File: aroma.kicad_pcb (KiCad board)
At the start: 4 copper layers, 96 x 44 mm, 108 parts, among them IC1 ESP32-WROOM-32E-N8R2, J1 USB4105-GF-A, J2 691137710003, J3 691137710002, J4 691137710002, J5 691137710002, J6 691137710002, J7 691137710002, J8 691137710002, J9 691137710002, Q1 SS8050, Q2 SS8050, SW1 1825910-6, SW2 1825910-6, SW3 JS5208, U1 FT231XS, U10 BSR802NL6327HTSA1, U11 BSR802NL6327HTSA1, U12 BSR802NL6327HTSA1, U2 ADP1613ARMZ-R7, U3 AMS1117-3.3, U4 74HC14, U6 BSR802NL6327HTSA1, U7 BSR802NL6327HTSA1, U8 BSR802NL6327HTSA1, U9 BSR802NL6327HTSA1

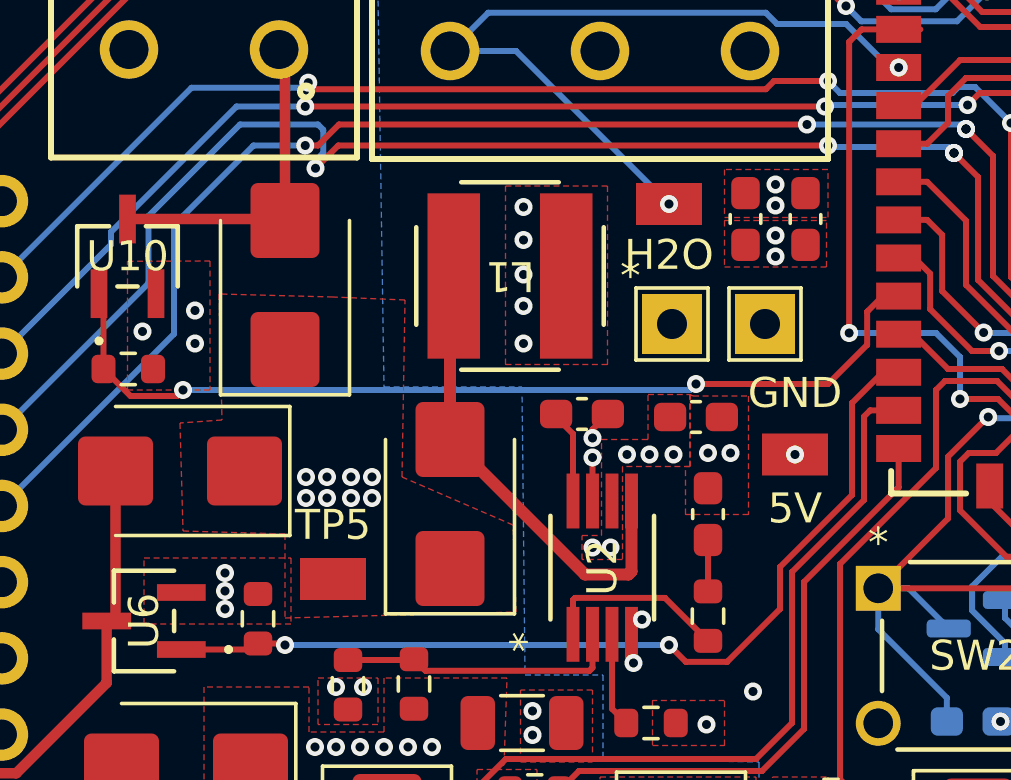
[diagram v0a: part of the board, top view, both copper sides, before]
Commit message: fix prelims
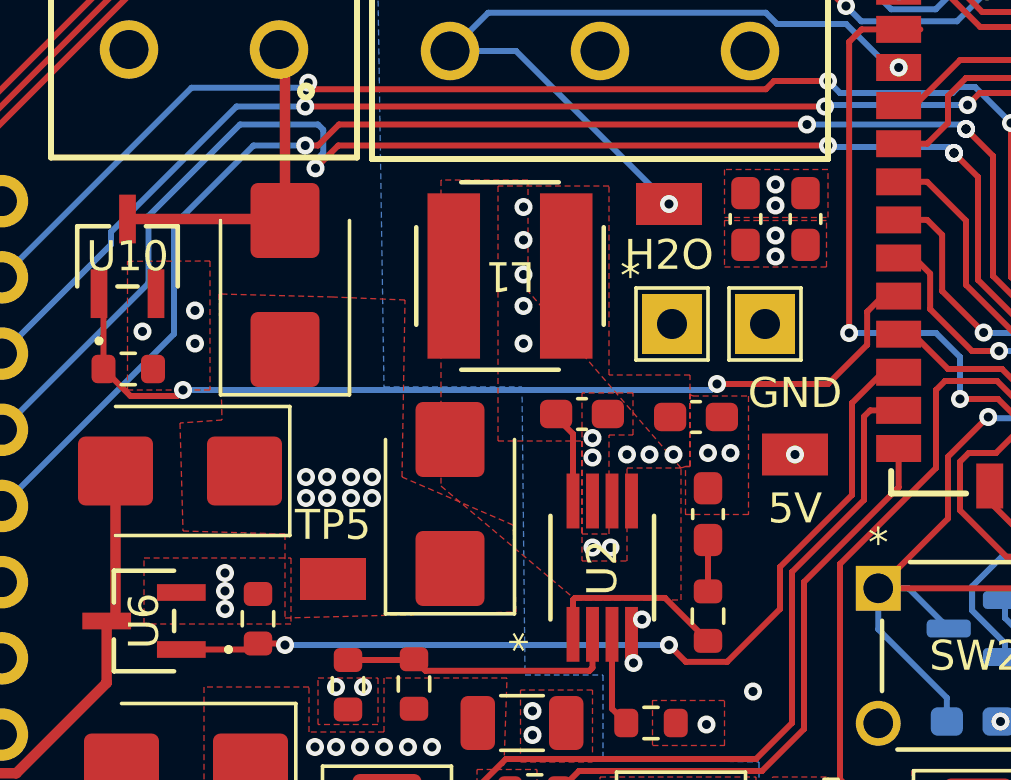
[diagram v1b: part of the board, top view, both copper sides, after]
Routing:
- net Net-(D4-A): track 15.8 -> 0.18 mm
- net GND: track 38.4 -> 35.9 mm
- added copper zone on F.Cu, net Net-(D4-A)
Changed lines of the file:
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@@
 	)
 	(segment
-		(start 138.65 96.45)
-		(end 138.65 97.899998)
-		(width 0.2)
-		(layer "F.Cu")
-		(net 1)
-	)
-	(segment
 		(start 126.250001 100.949999)
 		(end 126.4 100.8)
@@
 	)
 	(segment
-		(start 138.65 95.8)
-		(end 138.65 95.5125)
-		(width 0.2)
-		(layer "F.Cu")
-		(net 1)
-	)
-	(segment
 		(start 151.89 97.93)
 		(end 153.321299 99.361299)
@@
 	)
 	(segment
-		(start 138.65 95.5125)
-		(end 139.1625 95)
-		(width 0.2)
-		(layer "F.Cu")
-		(net 1)
-	)
-	(segment
 		(start 166.4875 100.860599)
 		(end 166.4875 102.6875)
@@
 	)
 	(segment
-		(start 133.9 95.85)
-		(end 133.9 90.525)
-		(width 0.4)
-		(layer "F.Cu")
-		(net 19)
-	)
-	(segment
-		(start 138.4 100.35)
-		(end 133.9 95.85)
-		(width 0.4)
-		(layer "F.Cu")
-		(net 19)
-	)
-	(segment
-		(start 139.949998 97.9)
-		(end 139.949998 100.250002)
-		(width 0.4)
-		(layer "F.Cu")
-		(net 19)
-	)
-	(segment
-		(start 139.85 100.35)
-		(end 138.4 100.35)
-		(width 0.4)
-		(layer "F.Cu")
-		(net 19)
-	)
-	(segment
 		(start 133.9 90.525)
 		(end 134.025 90.4)
@@
 	)
 	(segment
-		(start 139.949998 100.250002)
-		(end 139.85 100.35)
-		(width 0.4)
-		(layer "F.Cu")
-		(net 19)
-	)
-	(segment
 		(start 122.74 96.89)
 		(end 122.75 96.9)
@@
 	)
 	(segment
-		(start 142.1 94)
-		(end 146.5 94)
+		(start 125 94.2)
+		(end 124.8 94.4)
 		(width 0.2)
 		(layer "F.Cu")
@@
 	)
 	(segment
-		(start 125 94.2)
-		(end 124.8 94.4)
+		(start 147.805 92.695)
+		(end 147.805 91.59)
 		(width 0.2)
 		(layer "F.Cu")
@@
 	)
 	(segment
-		(start 147.805 91.59)
-		(end 148.325 91.07)
+		(start 142.8 94)
+		(end 146.5 94)
 		(width 0.2)
 		(layer "F.Cu")
@@
 	)
 	(segment
-		(start 124.8 94.4)
-		(end 123.25 94.4)
+		(start 147.805 91.59)
+		(end 148.325 91.07)
 		(width 0.2)
 		(layer "F.Cu")
@@
 	)
 	(segment
-		(start 148.325 91.07)
-		(end 148.855 91.07)
+		(start 124.8 94.4)
+		(end 123.25 94.4)
 		(width 0.2)
 		(layer "F.Cu")
@@
 	)
 	(segment
-		(start 122.35 91.1392)
-		(end 122.2 90.9892)
+		(start 146.5 94)
+		(end 147.805 92.695)
 		(width 0.2)
 		(layer "F.Cu")
@@
 	)
 	(segment
-		(start 147.805 92.695)
-		(end 147.805 91.59)
+		(start 122.35 91.1392)
+		(end 122.2 90.9892)
 		(width 0.2)
 		(layer "F.Cu")
@@
 	)
 	(segment
-		(start 146.5 94)
-		(end 147.805 92.695)
+		(start 148.325 91.07)
+		(end 148.855 91.07)
 		(width 0.2)
 		(layer "F.Cu")
@@
 	)
 	(via
-		(at 142.1 94)
+		(at 142.8 94)
 		(size 0.6)
 		(drill 0.3)
@@
 	)
 	(segment
-		(start 142.1 94)
-		(end 141.9 94.2)
+		(start 142.8 94)
+		(end 142.6 94.2)
 		(width 0.2)
 		(layer "B.Cu")
@@
 	)
 	(segment
-		(start 141.9 94.2)
+		(start 142.6 94.2)
 		(end 125 94.2)
 		(width 0.2)
@@
 	)
 	(zone
+		(net 1)
+		(net_name "GND")
+		(layer "F.Cu")
+		(hatch edge 0.5)
+		(priority 2)
+		(connect_pads yes
+			(clearance 0.25)
+		)
+		(min_thickness 0.25)
+		(filled_areas_thickness no)
+		(fill yes
+			(thermal_gap 0.5)
+			(thermal_bridge_width 0.5)
+		)
+		(polygon
+			(pts
+				(xy 140 94.3) (xy 138.3 94.3) (xy 138.3 99) (xy 139.2 99) (xy 139.2 95.7) (xy 140 95.7)
+			)
+		)
+	)
+	(zone
 		(net 6)
 		(net_name "+5V")
@@
 	)
 	(zone
-		(net 6)
-		(net_name "+5V")
-		(layer "F.Cu")
-		(hatch edge 0.5)
-		(priority 16)
-		(connect_pads yes
-			(clearance 0.25)
-		)
-		(min_thickness 0.2)
-		(filled_areas_thickness no)
-		(fill yes
-			(thermal_gap 0.5)
-			(thermal_bridge_width 0.5)
-		)
-		(polygon
-			(pts
-				(xy 135.75 87.4) (xy 139.15 87.4) (xy 139.15 93.35) (xy 135.75 93.35)
-			)
-		)
-	)
-	(zone
 		(net 1)
 		(net_name "GND")
@@
 	)
 	(zone
+		(net 19)
+		(net_name "Net-(D4-A)")
+		(layer "F.Cu")
+		(hatch edge 0.5)
+		(priority 1)
+		(connect_pads yes
+			(clearance 0.25)
+		)
+		(min_thickness 0.25)
+		(filled_areas_thickness no)
+		(fill yes
+			(thermal_gap 0.5)
+			(thermal_bridge_width 0.5)
+		)
+		(polygon
+			(pts
+				(xy 133.6 87.2) (xy 133.6 97.4) (xy 138.1 101.2) (xy 141.6 101.2) (xy 141.6 96.8) (xy 136.5 90.9)
+				(xy 136.5 87.2)
+			)
+		)
+	)
+	(zone
 		(net 1)
 		(net_name "GND")
@@
 		(layer "F.Cu")
 		(hatch edge 0.5)
-		(priority 17)
+		(priority 16)
 		(connect_pads yes
 			(clearance 0.25)
 		)
-		(min_thickness 0.2)
+		(min_thickness 0.25)
 		(filled_areas_thickness no)
 		(fill yes
@@
 		(polygon
 			(pts
-				(xy 139.65 95.85) (xy 140.5 95.85) (xy 140.5 94.35) (xy 141.9 94.35) (xy 141.9 96.75) (xy 139.65 96.75)
-				(xy 139.65 99.85) (xy 138.3 99.85) (xy 138.3 99.05) (xy 138.95 99.05) (xy 138.95 95.85)
+				(xy 139.2 87.4) (xy 135.5 87.4) (xy 135.5 95.9) (xy 138.3 95.9) (xy 138.3 99.9) (xy 139.8 99.9)
+				(xy 139.8 96.8) (xy 141.6 96.8) (xy 141.75 96.75) (xy 141.9 96.75) (xy 141.9 93.7) (xy 139.2 93.7)
 			)
 		)
